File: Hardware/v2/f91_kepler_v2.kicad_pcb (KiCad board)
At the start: 4 copper layers, 25 x 27 mm, 89 parts, among them J1 LS013B7DH03 FPC, Q1 FS8205A, SW1 BTN1/BSL, SW2 BTN2, SW3 BTN3, U1 CC2652R7RGZ, U2 BQ51050B, U3 DW01A, U4 XC6206P302MR, U5 LIS2DW12, U6 DRV2605L, U7 ST25DV04K, Y1 48MHz FA-128, Y2 32.768kHz FC-135

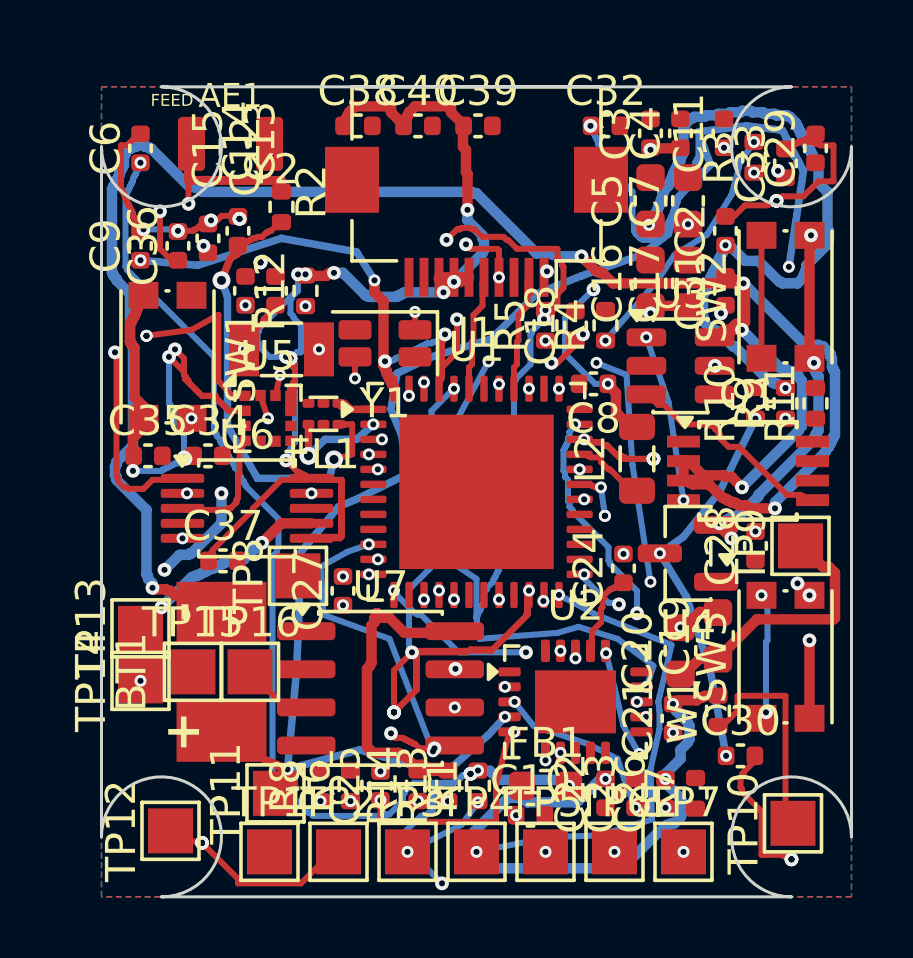
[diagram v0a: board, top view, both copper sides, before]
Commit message: wip: snapshot pre-migración
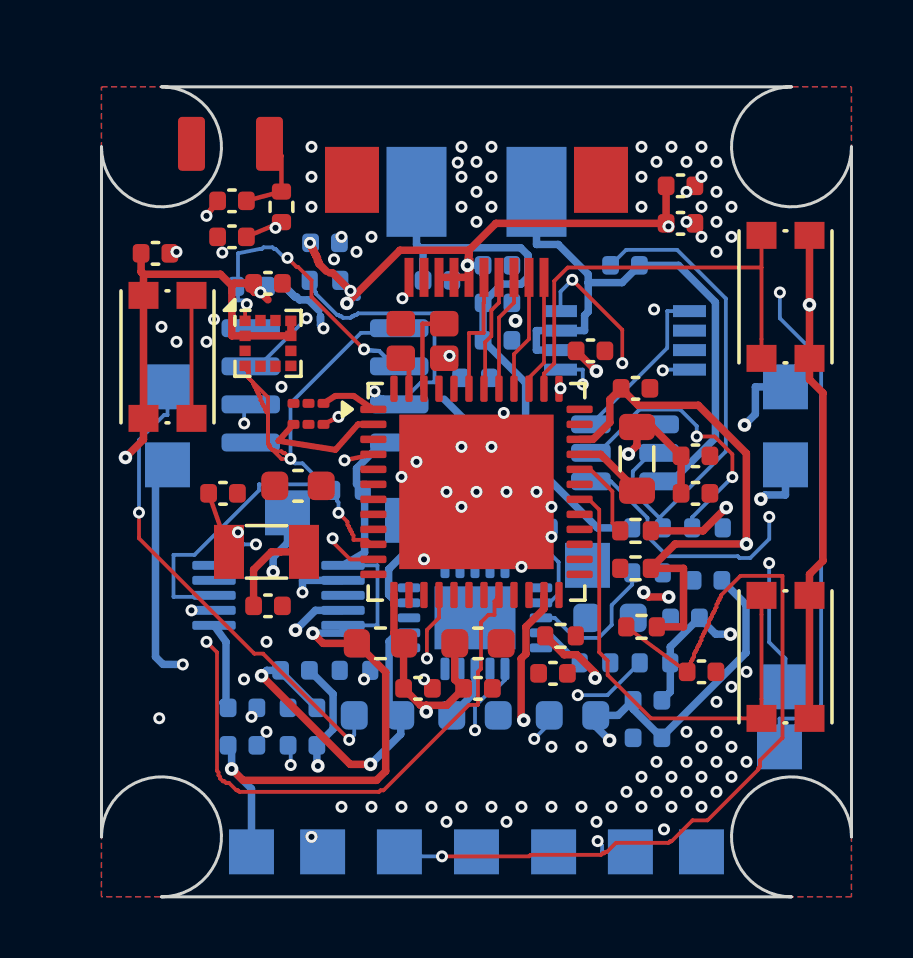
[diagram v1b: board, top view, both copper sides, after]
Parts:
- BT1: footprint f91_footprints:BatteryPads -> f91_footprints:Back_BatteryPads; moved to B.Cu
- C16, C17, C19, C20: footprint Capacitor_SMD:C_0603_1608Metric -> f91_footprints:Back_C_0603_1608Metric; moved to B.Cu
- C18, C21, C22, C23, C24, C25, C26, C27, C28, C29, C30, C31, C32, C33, C36, C37, C38: footprint Capacitor_SMD:C_0402_1005Metric -> f91_footprints:Back_C_0402_1005Metric; moved to B.Cu
- FL1: footprint f91_footprints:Murata_LFB18_1608 -> f91_footprints:F91_Murata_LFB18_1608
- J1: footprint Connector_FFC-FPC:Hirose_FH12-10S-0.5SH_1x10-1MP_P0.50mm_Horizontal -> f91_footprints:F91_LCD_FPC_Hirose_FH12-10
- Q1: footprint Package_SO:TSSOP-8_3x3mm_P0.65mm -> f91_footprints:Back_TSSOP-8_3x3mm_P0.65mm; moved to B.Cu
- R10, R11, R12, R13, R14, R5, R6, R7, R8, W1: footprint Resistor_SMD:R_0402_1005Metric -> f91_footprints:Back_R_0402_1005Metric; moved to B.Cu
- TP1, TP10, TP11, TP12, TP13, TP14, TP15, TP16, TP2, TP3, TP4, TP5, TP6, TP7, TP8, TP9: footprint TestPoint:TestPoint_Pad_1.5x1.5mm -> f91_footprints:Back_TestPoint_Pad_1.5x1.5mm; moved to B.Cu
- U2: footprint f91_footprints:VQFN-20-1EP_4.5x3.5mm_P0.5mm -> f91_footprints:Back_VQFN-20-1EP_4.5x3.5mm_P0.5mm; moved to B.Cu
- U3: footprint Package_TO_SOT_SMD:SOT-23-6 -> f91_footprints:Back_SOT-23-6; moved to B.Cu
- U4: footprint Package_TO_SOT_SMD:SOT-23 -> f91_footprints:Back_SOT-23; moved to B.Cu
- U6: footprint f91_footprints:VSSOP-10_3x3mm_P0.5mm -> f91_footprints:Back_VSSOP-10_3x3mm_P0.5mm; moved to B.Cu
- U7: footprint Package_SO:SOIC-8_3.9x4.9mm_P1.27mm -> f91_footprints:Back_SOIC-8_3.9x4.9mm_P1.27mm; moved to B.Cu
- Y1: footprint f91_footprints:Crystal_SMD_3215-4Pin_3.2x1.5mm -> f91_footprints:Epson_FA-128_2.0x1.6mm
- moved TP10 24.0 mm to (2.20, 12.6), turned to 0 degrees
- moved TP13 23.0 mm to (22.8, 10.0), turned to 0 degrees
- moved TP14 22.7 mm to (22.8, 12.6), turned to 0 degrees
- moved TP9 21.8 mm to (2.20, 10.0), turned to 0 degrees
- moved C6 20.2 mm to (10.6, 20.1), turned to 0 degrees
- moved C9 19.8 mm to (19.8, 12.3), turned to 0 degrees
- moved TP15 19.8 mm to (22.8, 20.0)
- moved C3 19.4 mm to (12.6, 20.1), turned to 0 degrees
- moved C4 18.5 mm to (15.1, 19.6), turned to 0 degrees
- moved BT1 18.1 mm to (12.5, 3.50), turned to 0 degrees
- moved C11 18.0 mm to (20.0, 19.5), turned to 0 degrees
- moved TP16 17.8 mm to (22.6, 22.0)
- moved R14 17.6 mm to (5.00, 6.65), turned to 0 degrees
- moved C30 17.1 mm to (13.2, 7.20)
- moved TP12 16.5 mm to (16.2, 15.9), turned to 0 degrees
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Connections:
- U1 pad 39: LCD_EXTCOMIN -> LCD_SCLK
- U1 pad 41: LCD_SCLK -> LCD_CS
- U1 pad 42: LCD_CS -> LCD_EXTCOMIN
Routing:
- net VDDS: track 155.7 -> 38.8 mm, vias 21 -> 2
- net FOD_TAP: track 66.2 -> 1.70 mm, vias 6 -> 0
- net VBAT: track 85.0 -> 28.2 mm, vias 7 -> 0
- net BATN: track 68.6 -> 20.9 mm, vias 6 -> 0
- net NFC_GPO: track 2.90 -> 42.2 mm, vias 3 -> 2
- net NFC_B: track 2.37 -> 39.4 mm, vias 0 -> 2
- net VDDR: track 40.2 -> 7.01 mm, vias 8 -> 1
- net NFC_A: track 0.00 -> 32.4 mm, vias 0 -> 2
- net UART_TX: track 0.00 -> 29.3 mm
- net DCOUPL: track 0.00 -> 28.6 mm
- net GND: track 29.0 -> 2.26 mm, vias 13 -> 107
- net AC2: track 20.8 -> 43.9 mm, vias 6 -> 2
- net PIEZO: track 8.45 -> 29.5 mm, vias 2 -> 5
- net SWD_TCK: track 20.1 -> 0.00 mm, vias 3 -> 0
- net CHG_DET: track 17.7 -> 0.00 mm, vias 5 -> 0
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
